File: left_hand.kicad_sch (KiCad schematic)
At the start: 54 parts

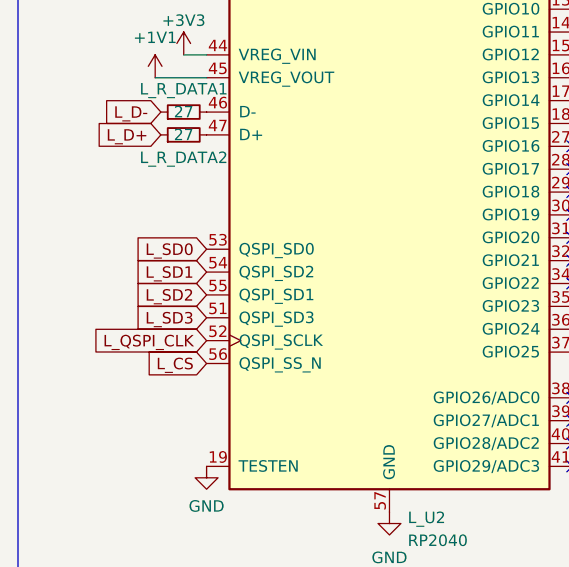
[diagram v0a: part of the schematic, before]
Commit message: final, working
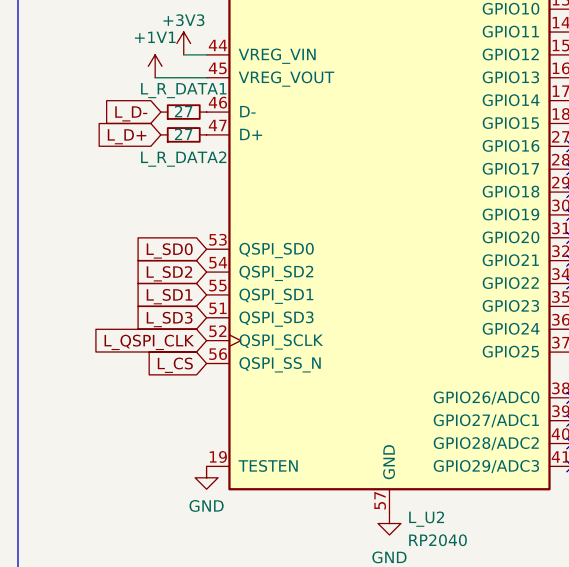
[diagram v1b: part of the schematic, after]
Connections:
- net L_SD1: now also L_U2.55 (QSPI_SD1); no longer L_U2.54 (QSPI_SD2)
- net L_SD2: now also L_U2.54 (QSPI_SD2); no longer L_U2.55 (QSPI_SD1)

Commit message: replace trrs
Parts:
- MX19, MX20, MX21, MX22, MX23, MX24, MX25, MX26, MX27, MX28, MX29, MX30, MX31, MX32, MX33, MX34, MX35, MX36: footprint parts:mx_1u -> parts:Kailh_socket_MX
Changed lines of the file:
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@@
       (effects (font (size 1.27 1.27)))
     )
-    (property "Footprint" "parts:mx_1u" (at 224.79 85.725 0)
+    (property "Footprint" "parts:Kailh_socket_MX" (at 224.79 85.725 0)
       (effects (font (size 1.27 1.27)) hide)
     )
@@
       (effects (font (size 1.27 1.27)))
     )
-    (property "Footprint" "parts:mx_1u" (at 173.99 28.575 0)
+    (property "Footprint" "parts:Kailh_socket_MX" (at 173.99 28.575 0)
       (effects (font (size 1.27 1.27)) hide)
     )
@@
       (effects (font (size 1.27 1.27)))
     )
-    (property "Footprint" "parts:mx_1u" (at 199.39 28.575 0)
+    (property "Footprint" "parts:Kailh_socket_MX" (at 199.39 28.575 0)
       (effects (font (size 1.27 1.27)) hide)
     )
@@
       (effects (font (size 1.27 1.27)))
     )
-    (property "Footprint" "parts:mx_1u" (at 199.39 66.675 0)
+    (property "Footprint" "parts:Kailh_socket_MX" (at 199.39 66.675 0)
       (effects (font (size 1.27 1.27)) hide)
     )
@@
       (effects (font (size 1.27 1.27)))
     )
-    (property "Footprint" "parts:mx_1u" (at 173.99 47.625 0)
+    (property "Footprint" "parts:Kailh_socket_MX" (at 173.99 47.625 0)
       (effects (font (size 1.27 1.27)) hide)
     )
@@
       (effects (font (size 1.27 1.27)))
     )
-    (property "Footprint" "parts:mx_1u" (at 186.69 66.675 0)
+    (property "Footprint" "parts:Kailh_socket_MX" (at 186.69 66.675 0)
       (effects (font (size 1.27 1.27)) hide)
     )
@@
       (effects (font (size 1.27 1.27)))
     )
-    (property "Footprint" "parts:mx_1u" (at 186.69 47.625 0)
+    (property "Footprint" "parts:Kailh_socket_MX" (at 186.69 47.625 0)
       (effects (font (size 1.27 1.27)) hide)
     )
@@
       (effects (font (size 1.27 1.27)))
     )
-    (property "Footprint" "parts:mx_1u" (at 212.09 28.575 0)
+    (property "Footprint" "parts:Kailh_socket_MX" (at 212.09 28.575 0)
       (effects (font (size 1.27 1.27)) hide)
     )
@@
       (effects (font (size 1.27 1.27)))
     )
-    (property "Footprint" "parts:mx_1u" (at 199.39 85.725 0)
+    (property "Footprint" "parts:Kailh_socket_MX" (at 199.39 85.725 0)
       (effects (font (size 1.27 1.27)) hide)
     )
@@
       (effects (font (size 1.27 1.27)))
     )
-    (property "Footprint" "parts:mx_1u" (at 212.09 47.625 0)
+    (property "Footprint" "parts:Kailh_socket_MX" (at 212.09 47.625 0)
       (effects (font (size 1.27 1.27)) hide)
     )
@@
       (effects (font (size 1.27 1.27)))
     )
-    (property "Footprint" "parts:mx_1u" (at 212.09 85.725 0)
+    (property "Footprint" "parts:Kailh_socket_MX" (at 212.09 85.725 0)
       (effects (font (size 1.27 1.27)) hide)
     )
@@
       (effects (font (size 1.27 1.27)))
     )
-    (property "Footprint" "parts:mx_1u" (at 186.69 28.575 0)
+    (property "Footprint" "parts:Kailh_socket_MX" (at 186.69 28.575 0)
       (effects (font (size 1.27 1.27)) hide)
     )
@@
       (effects (font (size 1.27 1.27)))
     )
-    (property "Footprint" "parts:mx_1u" (at 224.79 28.575 0)
+    (property "Footprint" "parts:Kailh_socket_MX" (at 224.79 28.575 0)
       (effects (font (size 1.27 1.27)) hide)
     )
@@
       (effects (font (size 1.27 1.27)))
     )
-    (property "Footprint" "parts:mx_1u" (at 224.79 66.675 0)
+    (property "Footprint" "parts:Kailh_socket_MX" (at 224.79 66.675 0)
       (effects (font (size 1.27 1.27)) hide)
     )
@@
       (effects (font (size 1.27 1.27)))
     )
-    (property "Footprint" "parts:mx_1u" (at 173.99 66.675 0)
+    (property "Footprint" "parts:Kailh_socket_MX" (at 173.99 66.675 0)
       (effects (font (size 1.27 1.27)) hide)
     )
@@
       (effects (font (size 1.27 1.27)))
     )
-    (property "Footprint" "parts:mx_1u" (at 212.09 66.675 0)
+    (property "Footprint" "parts:Kailh_socket_MX" (at 212.09 66.675 0)
       (effects (font (size 1.27 1.27)) hide)
     )
@@
       (effects (font (size 1.27 1.27)))
     )
-    (property "Footprint" "parts:mx_1u" (at 224.79 47.625 0)
+    (property "Footprint" "parts:Kailh_socket_MX" (at 224.79 47.625 0)
       (effects (font (size 1.27 1.27)) hide)
     )
@@
       (effects (font (size 1.27 1.27)))
     )
-    (property "Footprint" "parts:mx_1u" (at 199.39 47.625 0)
-      (effects (font (size 1.27 1.27)) hide)
-    )
+    (property "Footprint" "parts:Kailh_socket_MX" (at 199.39 47.625 0)
+      (effects (font (size 1.27 1.27)) hide)
+    )
